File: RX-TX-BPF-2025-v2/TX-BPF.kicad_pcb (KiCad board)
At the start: 11 copper layers, 60.6 x 26.8 mm, 21 parts

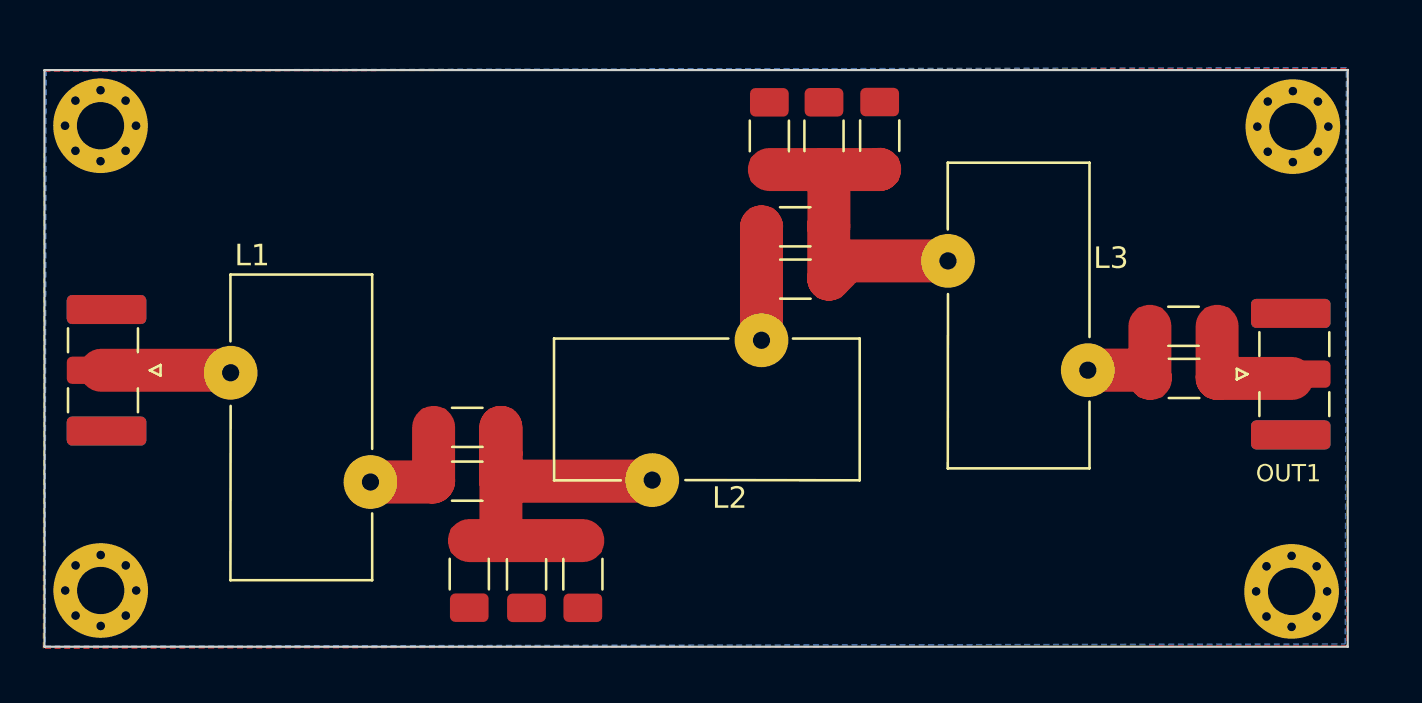
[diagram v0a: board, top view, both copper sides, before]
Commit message: A new start...
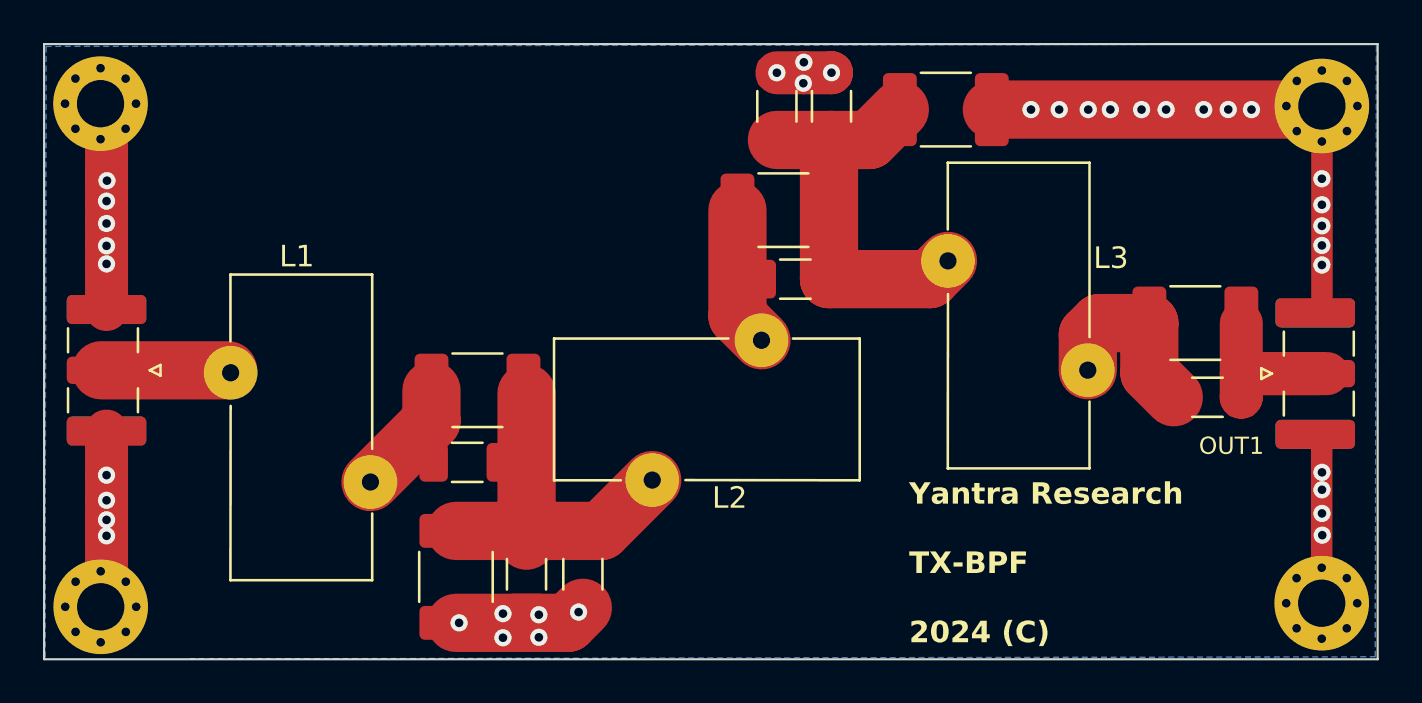
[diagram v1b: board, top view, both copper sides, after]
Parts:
- CFL3, CFS2, CSL2, CSS1, CTS2: footprint Capacitor_SMD:C_1206_3216Metric_Pad1.33x1.80mm_HandSolder -> Capacitor_SMD:C_1812_4532Metric_Pad1.57x3.40mm_HandSolder
- moved CSL2 3.31 mm to (127.2, 85.7), turned to 0 degrees
- moved CFS2 1.79 mm to (105.5, 98.8)
- moved H2 1.66 mm to (144.7, 85.6)
- moved H3 1.50 mm to (144.7, 108.7)
- moved CSL3 1.42 mm to (121.9, 85.6)
- moved CSL1 1.42 mm to (119.4, 85.6)
- moved CTS1 1.40 mm to (139.4, 99.1)
- moved OUT1 1.14 mm to (144.7, 98.0)
- moved H1 1.02 mm to (88.0, 85.5)
- moved CSS1 0.95 mm to (119.7, 90.4)
- moved CFS1 0.88 mm to (105.0, 102.1)
- moved H4 0.76 mm to (88.0, 108.8)
- moved CFL3 0.63 mm to (104.5, 107.5)
- moved CTS2 0.57 mm to (138.8, 95.7)
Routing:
- net GND: track 0.00 -> 58.6 mm, vias 0 -> 37
- net Net-(OUT1-In): track 5.89 -> 11.1 mm
- net Net-(CTS1-Pad1): track 5.47 -> 8.66 mm
- net Net-(CFL1-Pad1): track 20.0 -> 17.0 mm
- net Net-(CSL1-Pad1): track 16.1 -> 18.7 mm
- net Net-(CSS1-Pad1): track 5.28 -> 6.51 mm
- removed copper zone on F.Cu, net GND
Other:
- board size 60.6 x 26.8 mm -> 62 x 28.6 mm
- board text added: "Yantra Research TX-BPF 2024 (C)"
